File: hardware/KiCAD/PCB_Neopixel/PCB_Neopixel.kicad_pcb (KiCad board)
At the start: 2 copper layers, 124.5 x 10 mm, 54 parts, among them J1001 Conn_01x01, J1002 Conn_01x01, J1003 Conn_01x01, J101 Conn_01x01, J102 Conn_01x01, J103 Conn_01x01, J1101 Conn_01x01, J1102 Conn_01x01, J1103 Conn_01x01, J201 Conn_01x01, J202 Conn_01x01, J203 Conn_01x01, J301 Conn_01x01, J302 Conn_01x01, J303 Conn_01x01, J401 Conn_01x01, J402 Conn_01x01, J403 Conn_01x01, J501 Conn_01x01, J502 Conn_01x01, J503 Conn_01x01, J601 Conn_01x01, J602 Conn_01x01, J603 Conn_01x01, J701 Conn_01x01, J702 Conn_01x01, J703 Conn_01x01, J801 Conn_01x01, J802 Conn_01x01, J803 Conn_01x01, J901 Conn_01x01, J902 Conn_01x01, J903 Conn_01x01

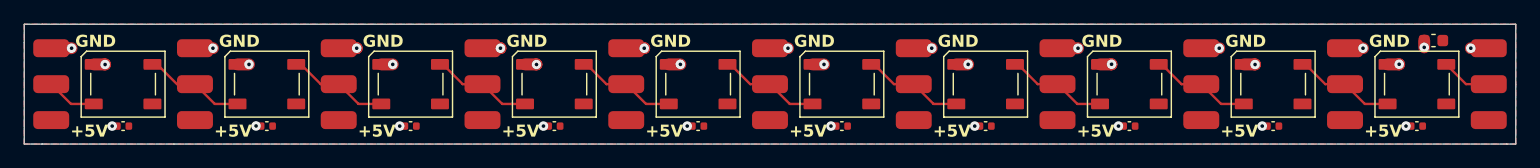
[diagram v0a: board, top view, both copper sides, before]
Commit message: PCB 100x10
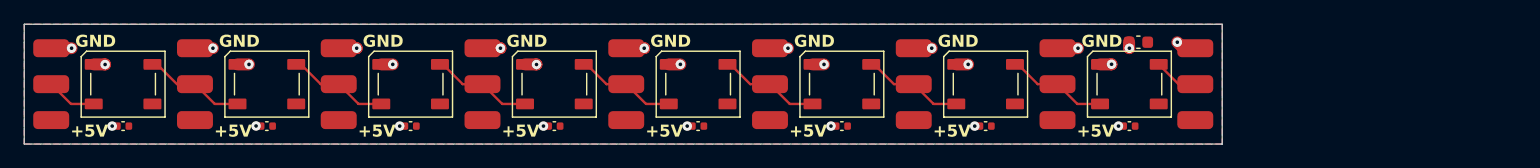
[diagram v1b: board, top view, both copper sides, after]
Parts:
- removed C1001, C1101: 100n, Capacitor_SMD:C_0402_1005Metric
- removed C101: 10u, Capacitor_SMD:C_0603_1608Metric
- removed D1001, D1101: WS2812B, LED_SMD:LED_WS2812B_PLCC4_5.0x5.0mm_P3.2mm
- removed J1001, J1002, J1003, J101, J102, J103, J1101, J1102, J1103: Conn_01x01, Connector_Wire:SolderWirePad_1x01_SMD_1.5x3mm
- added C1201: 10u, Capacitor_SMD:C_0603_1608Metric, F.Cu at (184.2, 96.5)
- added J1201: Conn_01x01, Connector_Wire:SolderWirePad_1x01_SMD_1.5x3mm, F.Cu at (189.0, 103.0)
- added J1202: Conn_01x01, Connector_Wire:SolderWirePad_1x01_SMD_1.5x3mm, F.Cu at (189.0, 97.0)
- added J1203: Conn_01x01, Connector_Wire:SolderWirePad_1x01_SMD_1.5x3mm, F.Cu at (189.0, 100.0)
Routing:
- net DO9: track 8.47 -> 0.00 mm
- net GND: track 31.4 -> 25.8 mm, vias 32 -> 26
- net DO8: track 8.47 -> 3.83 mm
- net DO: track 4.23 -> 0.00 mm
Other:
- board size 124.5 x 10 mm -> 100 x 10 mm
